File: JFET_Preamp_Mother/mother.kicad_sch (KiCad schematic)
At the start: 14 parts, among them J101 Conn_01x02, J102 Conn_01x06_Socket, J103 Conn_01x06_Socket, Q101 AO3401A

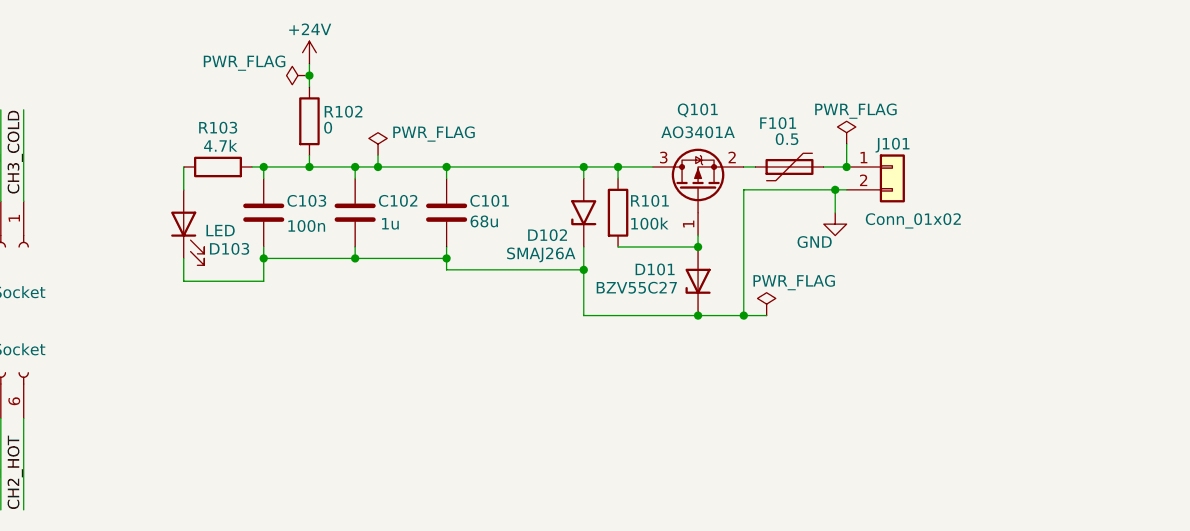
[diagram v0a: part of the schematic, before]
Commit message: push just to make sure everything is up to date
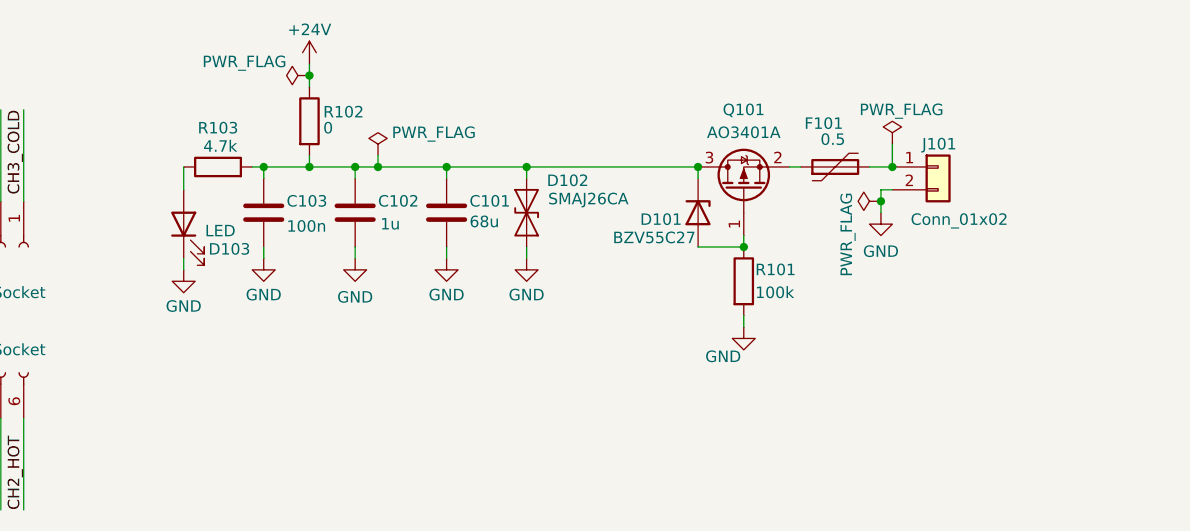
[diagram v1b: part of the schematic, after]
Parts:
- removed D102: SMAJ26A, Diode_SMD:D_SMA, symbol Diode:SMAJ26A
- added D102: SMAJ26CA, Diode_SMD:D_SMA, symbol Diode:SMAJ26CA
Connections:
- net GND: now also R101.2, D102.1 (A1); no longer D101.1 (K)
- net at C101.1, C102.1, C103.1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: now also D101.1 (K), D102.2 (A2); no longer R101.1
- net at D101.2 (A), Q101.1 (G): now also R101.1; no longer R101.2
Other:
- moved on the sheet: F101, J101, Q101
